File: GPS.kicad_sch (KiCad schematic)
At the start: 8 parts, among them J4 Conn_Coaxial, U2 NEO-6M-0-001

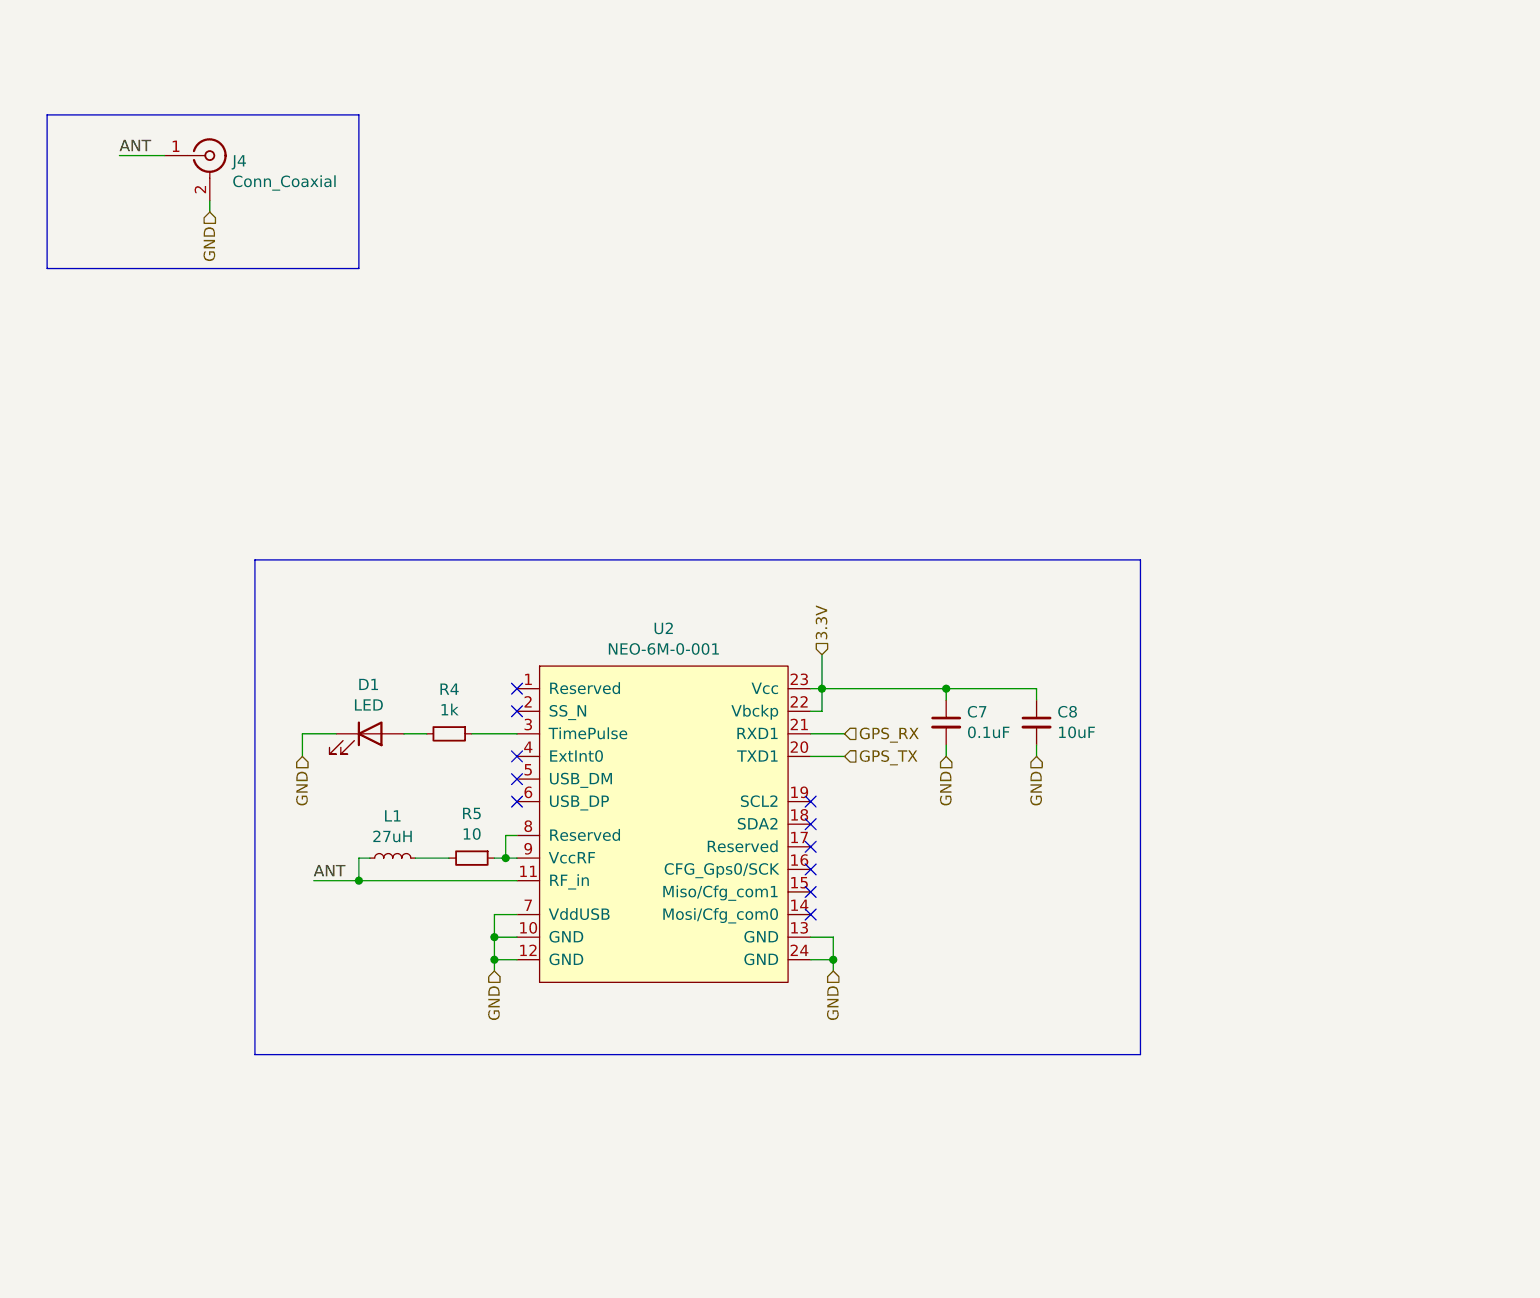
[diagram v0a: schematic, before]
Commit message: KiCad 0.2v
Schematics done.
Have to assign footprints to corresponding components.
Completely rework PCB.
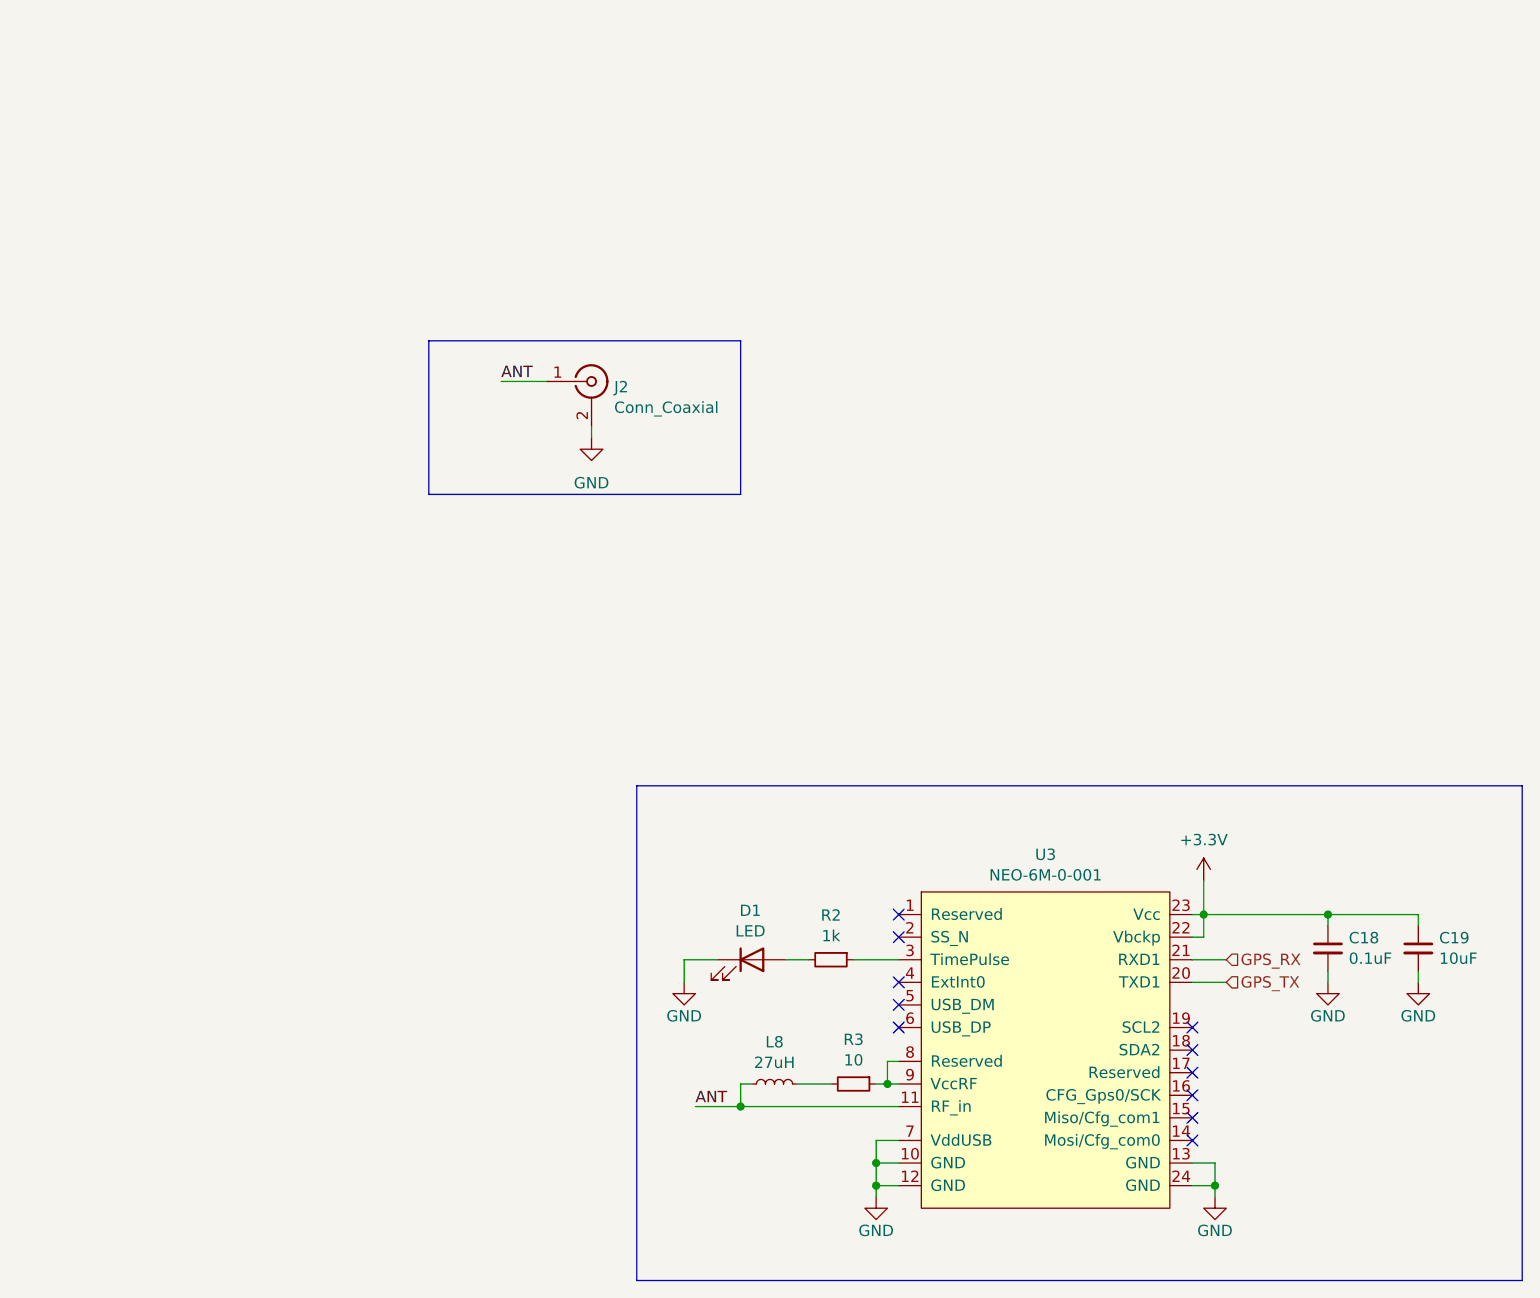
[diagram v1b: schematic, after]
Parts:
- removed C7: 0.1uF, Capacitor_SMD:C_0603_1608Metric, symbol Device:C_Small
- removed C8: 10uF, Capacitor_SMD:C_0603_1608Metric, symbol Device:C_Small
- removed J4: Conn_Coaxial, Connector_Coaxial:SMA_Amphenol_132134-16_Vertical, symbol Connector:Conn_Coaxial
- removed L1: 27uH, Capacitor_SMD:C_0805_2012Metric_Pad1.18x1.45mm_HandSolder, symbol Device:L_Small
- removed R4: 1k, Resistor_SMD:R_0603_1608Metric_Pad0.98x0.95mm_HandSolder, symbol Device:R_Small
- removed R5: 10, Capacitor_SMD:C_0603_1608Metric, symbol Device:R_Small
- removed U2: NEO-6M-0-001, footprints:XCVR_NEO-6M-GPS, symbol pastaisitie_simboli:NEO-6M-0-001
- added C18: 0.1uF, Capacitor_SMD:C_0603_1608Metric, symbol Device:C_Small
- added C19: 10uF, Capacitor_SMD:C_0603_1608Metric, symbol Device:C_Small
- added J2: Conn_Coaxial, Connector_Coaxial:SMA_Amphenol_132134-16_Vertical, symbol Connector:Conn_Coaxial
- added L8: 27uH, Capacitor_SMD:C_0805_2012Metric_Pad1.18x1.45mm_HandSolder, symbol Device:L_Small
- added R2: 1k, Resistor_SMD:R_0603_1608Metric_Pad0.98x0.95mm_HandSolder, symbol Device:R_Small
- added R3: 10, Capacitor_SMD:C_0603_1608Metric, symbol Device:R_Small
- added U3: NEO-6M-0-001, footprints:XCVR_NEO-6M-GPS, symbol pastaisitie_simboli:NEO-6M-0-001
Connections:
- net ANT: now also J2.1 (In), L8.1, U3.11 (RF_in)
- net GND: now also C18.2, C19.2, J2.2 (Ext), U3.10 (GND), U3.12 (GND), U3.13 (GND), U3.24 (GND), U3.7 (VddUSB)
- net GPS_RX: now also U3.21 (RXD1)
- net GPS_TX: now also U3.20 (TXD1)
- net at D1.2 (A): now also R2.2
- new net: R2.1, U3.3 (TimePulse)
- new net: R3.1, U3.8 (Reserved), U3.9 (VccRF)
- new net: L8.2, R3.2
- new net +3V3: C18.1, C19.1, U3.22 (Vbckp), U3.23 (Vcc)

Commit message: KiCad 0.3v
Improved aesthetics.
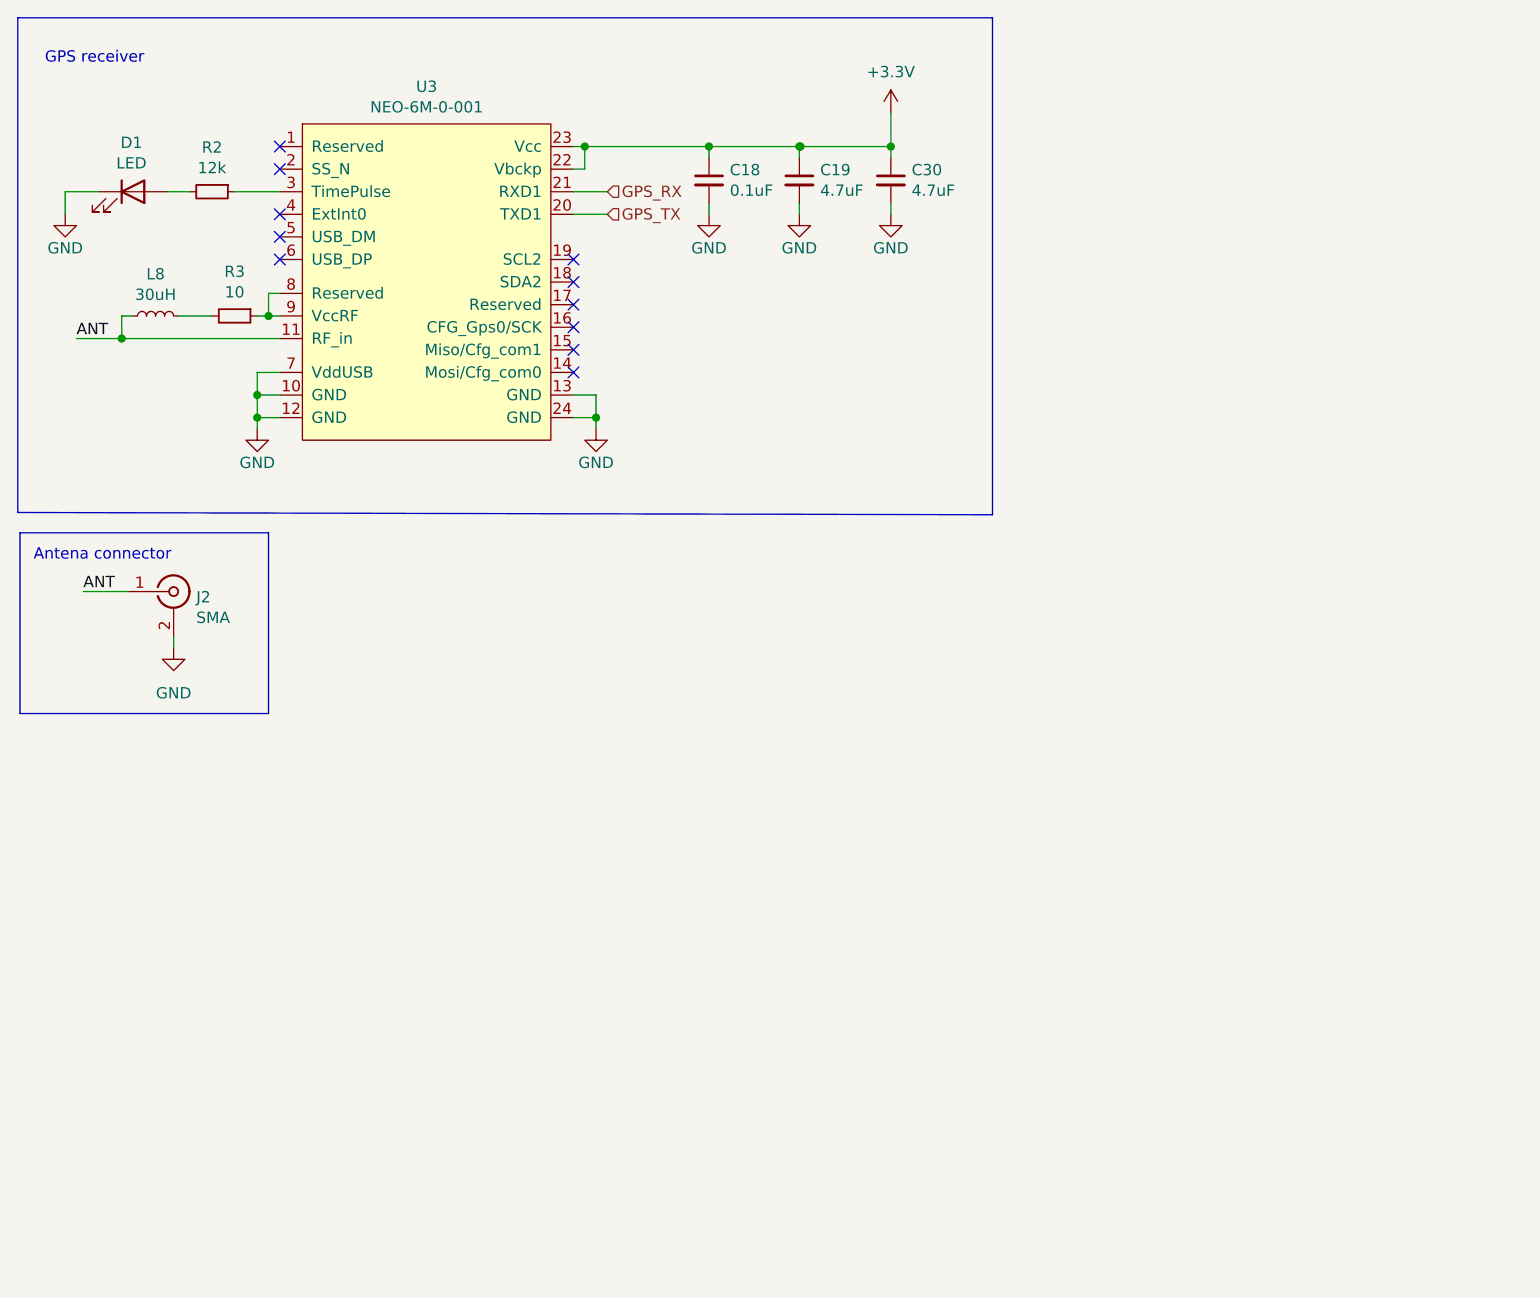
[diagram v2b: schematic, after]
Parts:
- added C30: 4.7uF, Capacitor_SMD:C_0603_1608Metric, symbol Device:C_Small
- C19: value 10uF -> 4.7uF
- J2: value Conn_Coaxial -> SMA
- L8: value 27uH -> 30uH
- R2: value 1k -> 12k
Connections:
- net +3V3: now also C30.1; no longer C18.1, C19.1, U3.22 (Vbckp), U3.23 (Vcc)
- net GND: now also C30.2
- new net: C18.1, C19.1, U3.22 (Vbckp), U3.23 (Vcc)
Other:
- note added: "Antena connector"
- note added: "GPS receiver"
- moved on the sheet: C18, C19, D1, J2, L8, R2, R3, U3

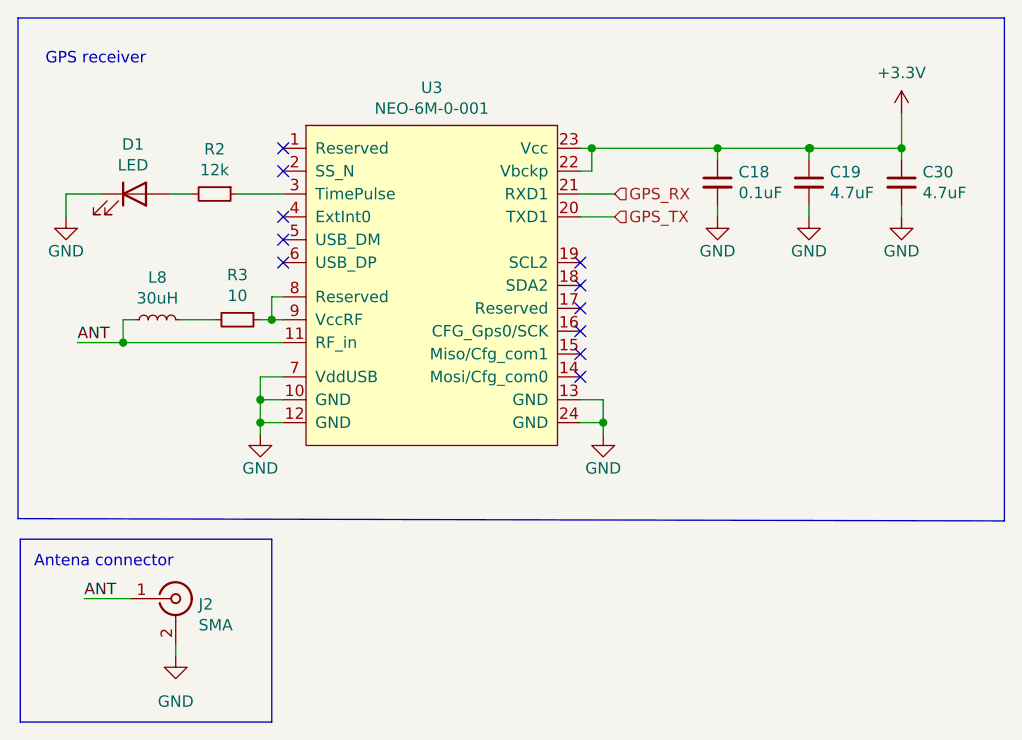
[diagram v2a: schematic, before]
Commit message: 0.1v COM_PCB KiCad
First iteration of COM PCB.
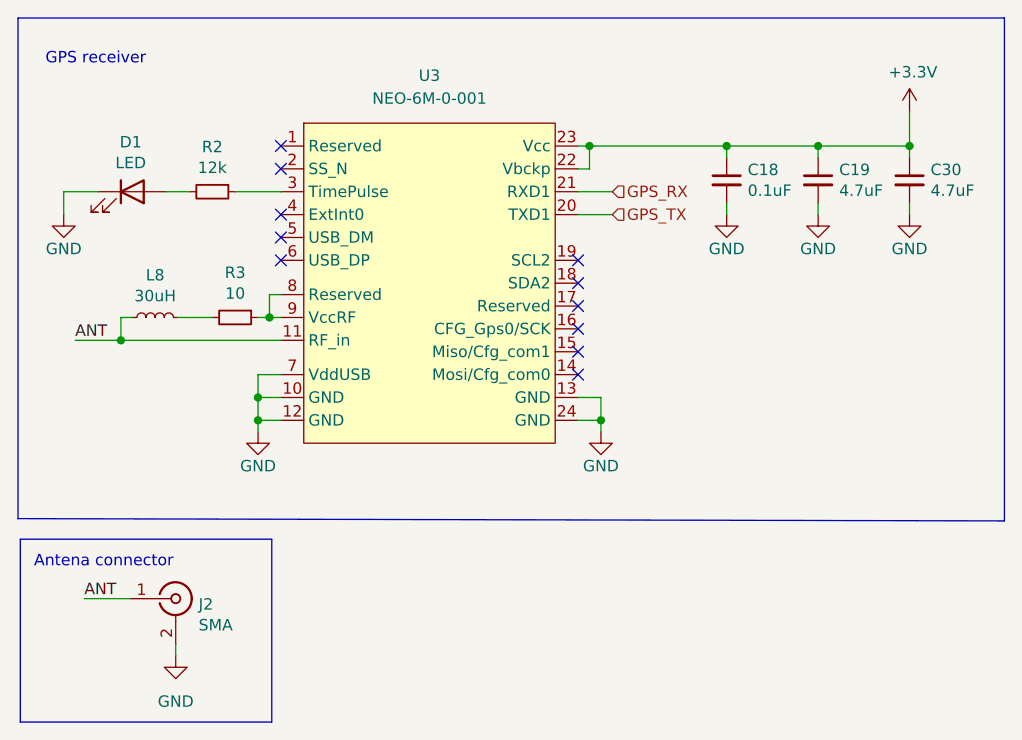
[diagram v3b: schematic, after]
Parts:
- removed U3: NEO-6M-0-001, footprints:XCVR_NEO-6M-GPS, symbol pastaisitie_simboli:NEO-6M-0-001
- added U3: NEO-6M-0-001, footprints:XCVR_NEO-6M-GPS, symbol schematics:NEO-6M-0-001
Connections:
- net +3V3: now also C18.1, C19.1, U3.22 (Vbckp), U3.23 (Vcc)
- net ANT: now also U3.11 (RF_in)
- net GND: now also U3.10 (GND), U3.12 (GND), U3.13 (GND), U3.24 (GND), U3.7 (VddUSB)
- net GPS_RX: now also U3.21 (RXD1)
- net GPS_TX: now also U3.20 (TXD1)
- net at R2.1: now also U3.3 (TimePulse)
- net at R3.1: now also U3.8 (Reserved), U3.9 (VccRF)
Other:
- moved on the sheet: C18, C19, C30

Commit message: V1
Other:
- company: (none) -> BASEMENT
- title: (none) -> GPS NEO-6N module
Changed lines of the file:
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@@
 (kicad_sch (version 20211123) (generator eeschema)
   (paper "A4")
+  (title_block
+    (title "GPS NEO-6N module")
+    (date "%%date%%")
+    (rev "%%version%%")
+    (company "BASEMENT")
+  )
   (junction (at 41.91 59.69) (diameter 0) (color 0 0 0 0)
   )
